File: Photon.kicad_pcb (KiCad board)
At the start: 4 copper layers, 22.4 x 95.8 mm, 58 parts, among them J1 USB_C_Receptacle_USB2.0_14P, Q1 IRLML6402, Q2 IRLML6402, SW1 TS-1088-AR02016, U1 ATtiny13A-S, U2 RT8059GJ5, U3 TP4056, U4 BCR421UW6-7, U5 DW01A, U6 FS8205A, U7 BCR421UW6-7

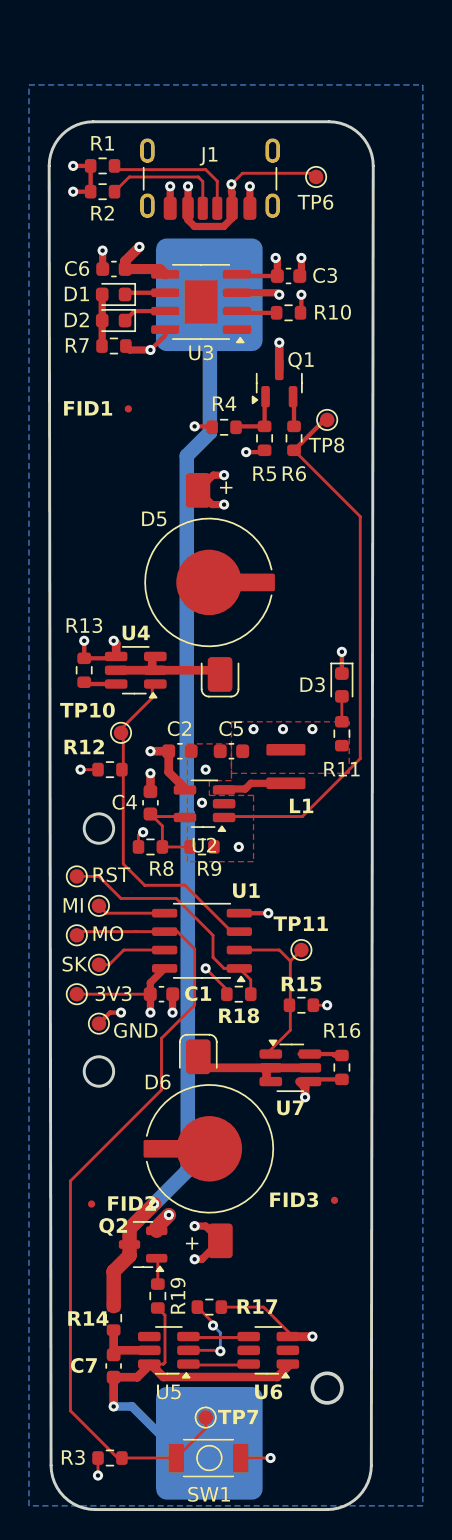
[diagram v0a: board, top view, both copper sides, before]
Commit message: finished v3 of pcb
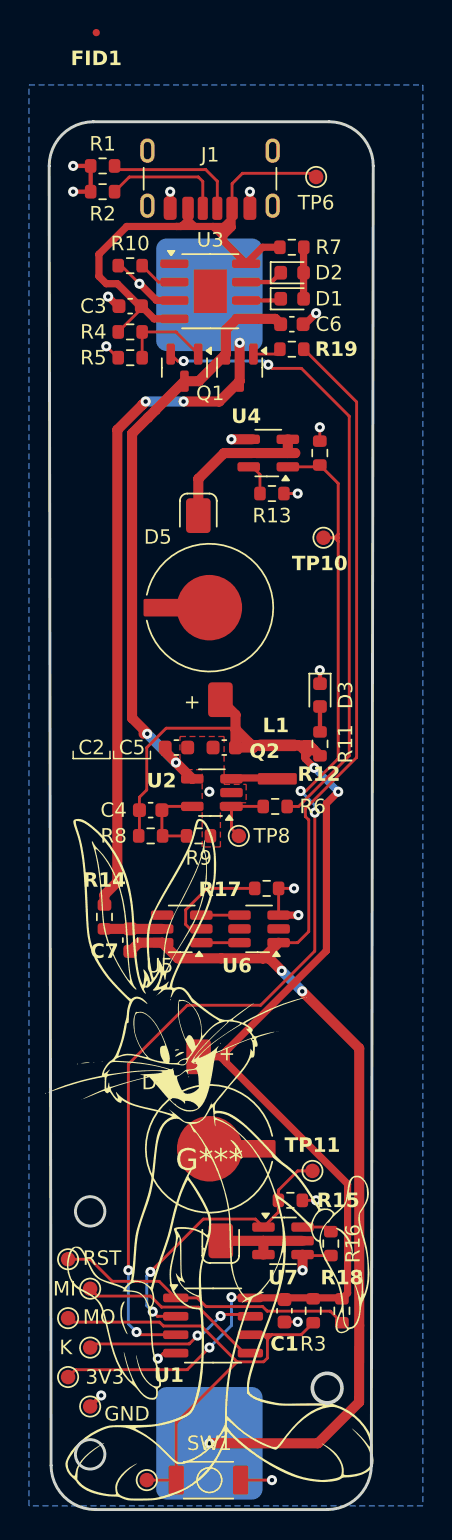
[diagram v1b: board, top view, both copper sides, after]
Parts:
- removed FID2, FID3: Fiducial, Fiducial:Fiducial_0.5mm_Mask1.5mm
- added G***: LOGO, Photon:Bugs_50mm, F.Cu at (52.8, 91.7)
- added G***: LOGO, Photon:bugs_side_40mm, B.Cu at (52.8, 61.8)
- moved R19 66.0 mm to (58.5, 35.8), turned to 0 degrees
- moved Q2 60.9 mm to (54.9, 37.0), turned to -90 degrees
- moved C7 29.4 mm to (47.4, 76.5)
- moved TP8 29.3 mm to (54.9, 69.3)
- moved R17 29.2 mm to (56.8, 73.0)
- moved U5 29.1 mm to (50.9, 75.8)
- moved U6 29.1 mm to (56.3, 75.8)
- moved R14 27.7 mm to (45.6, 74.9)
- moved U1 26.6 mm to (53.1, 103.1), turned to 0 degrees
- moved TP3 26.4 mm to (43.1, 98.6)
- moved TP9 26.4 mm to (43.1, 106.7)
- moved TP1 26.4 mm to (44.6, 108.7)
- moved TP2 26.4 mm to (44.6, 100.6)
- moved TP4 26.4 mm to (43.1, 102.6)
- moved TP5 26.4 mm to (44.6, 104.6)
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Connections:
- net /BAT_SAF_OUT renamed /Bat-
- net /PMOS_Gate renamed /USB_DSBL
- net /PMOS_OUT renamed /PMOS_EN_OUT
- net Net-(Q2-G) renamed /BAT_DSBL
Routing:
- net /Bat-: track 28.0 -> 102.2 mm, vias 1 -> 3
- net +3V3: track 23.5 -> 97.4 mm, vias 12 -> 4
- net /LED1_EN: track 23.2 -> 77.3 mm, vias 0 -> 4
- net /PMOS_EN_OUT: track 2.07 -> 43.3 mm, vias 0 -> 2
- net /BUCK_EN: track 37.8 -> 4.45 mm
- net PACK+: track 12.5 -> 41.6 mm, vias 4 -> 2
- net /Bat+: track 72.6 -> 45.7 mm, vias 1 -> 3
- net /MISO_BTN: track 56.4 -> 35.1 mm
- net 5V: track 23.4 -> 40.8 mm, vias 5 -> 0
- net GND: track 42.4 -> 32.9 mm, vias 23 -> 21
- net /MOSI: track 4.75 -> 12.9 mm
- net /LED2_EN: track 12.0 -> 20.1 mm, vias 0 -> 2
- net /SCK: track 4.96 -> 12.1 mm, vias 0 -> 2
- net /RESET: track 16.8 -> 20.7 mm
- net /OUT_LED1: track 7.99 -> 10.7 mm
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- added copper zone on B.Cu, net GND
- removed copper zone on F.Cu, net +3V3
- removed copper zone on In2.Cu, net +3V3
- removed copper zone on In2.Cu, net 5V
- removed copper zone on In1.Cu, net GND
- removed copper zone on B.Cu, net PACK+
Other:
- outline, holes or cut-outs redrawn
- copper layers 4 -> 2
- board text added: "K"
- board text removed: "SK"
